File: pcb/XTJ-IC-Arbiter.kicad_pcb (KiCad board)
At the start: 2 copper layers, 82.4 x 47.6 mm, 33 parts, among them J3 DTM13-12PA-R008, SW2 SW_DIP_x02, U1 LM2672N-5.0, U3 Teensy4.0, U4 MCP2562-H-P, U5 SP723ABG

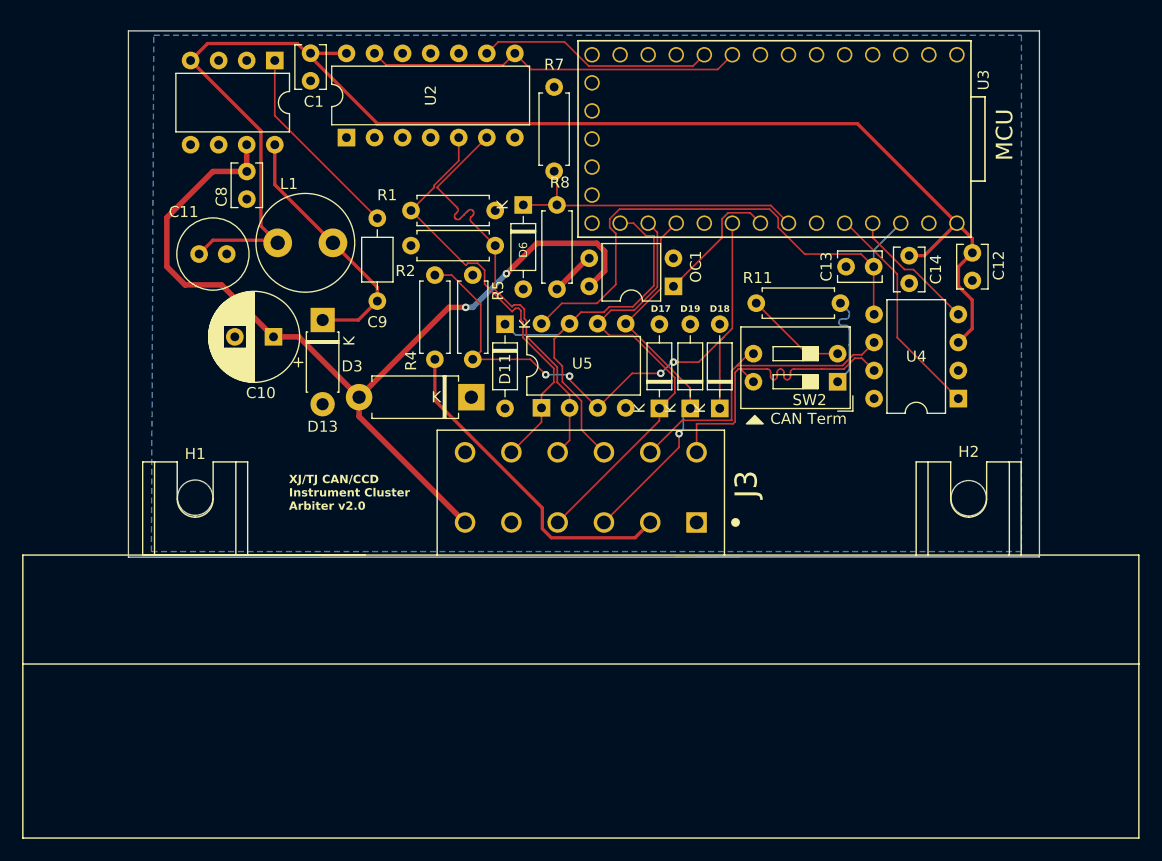
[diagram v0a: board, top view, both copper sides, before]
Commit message: fix board edge
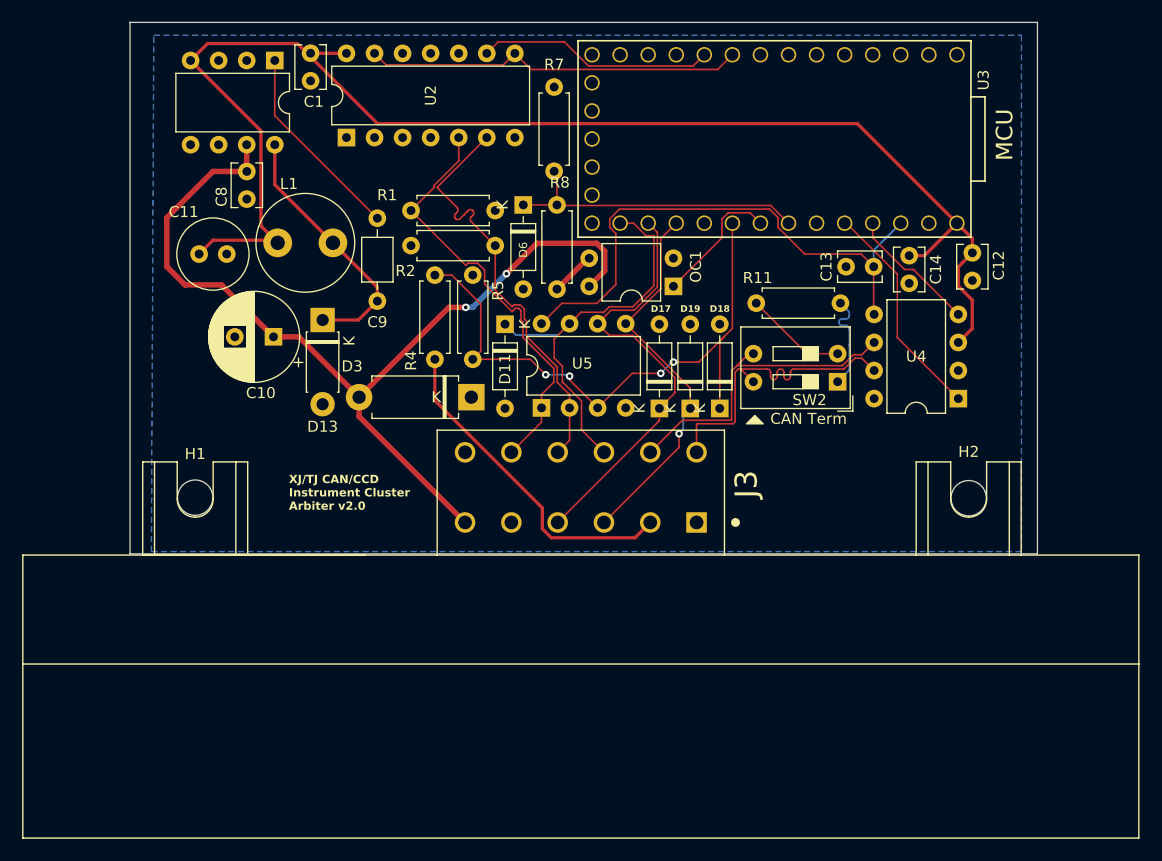
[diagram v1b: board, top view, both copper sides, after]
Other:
- board size 82.4 x 47.6 mm -> 82.1 x 48.1 mm
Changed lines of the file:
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@@
     )
     (stroke (width 0.12) (type solid)) (fill solid) (layer "F.SilkS"))
-  (gr_line (start 50.24 88.011) (end 132.69 88.011)
-    (stroke (width 0.05) (type default)) (layer "Edge.Cuts"))
-  (gr_line (start 50.244 135.64) (end 50.244 88.008)
-    (stroke (width 0.05) (type solid)) (layer "Edge.Cuts"))
-  (gr_line (start 132.69 88.011) (end 132.69 135.61)
-    (stroke (width 0.05) (type solid)) (layer "Edge.Cuts"))
-  (gr_line (start 132.69 135.61) (end 50.244 135.64)
-    (stroke (width 0.05) (type solid)) (layer "Edge.Cuts"))
+  (gr_rect (start 50.39 87.238) (end 132.51 135.338)
+    (stroke (width 0.05) (type default)) (fill none) (layer "Edge.Cuts"))
   (gr_text "CCD-\n" (at 88.6968 123.952) (layer "B.SilkS")
     (effects (font (size 1 1) (thickness 0.15)) (justify mirror))
